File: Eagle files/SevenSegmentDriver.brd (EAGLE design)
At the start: 18.4 x 25.4 mm, 4 parts, among them IC1 74HC595D

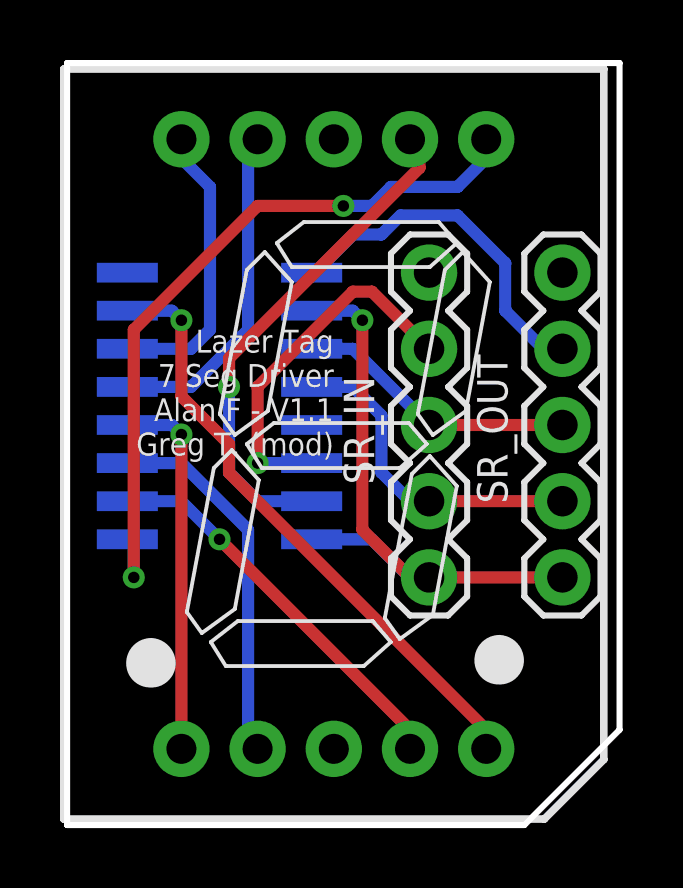
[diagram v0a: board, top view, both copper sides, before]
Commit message: Fixes
more fixes >:|
should e ready for fabbing
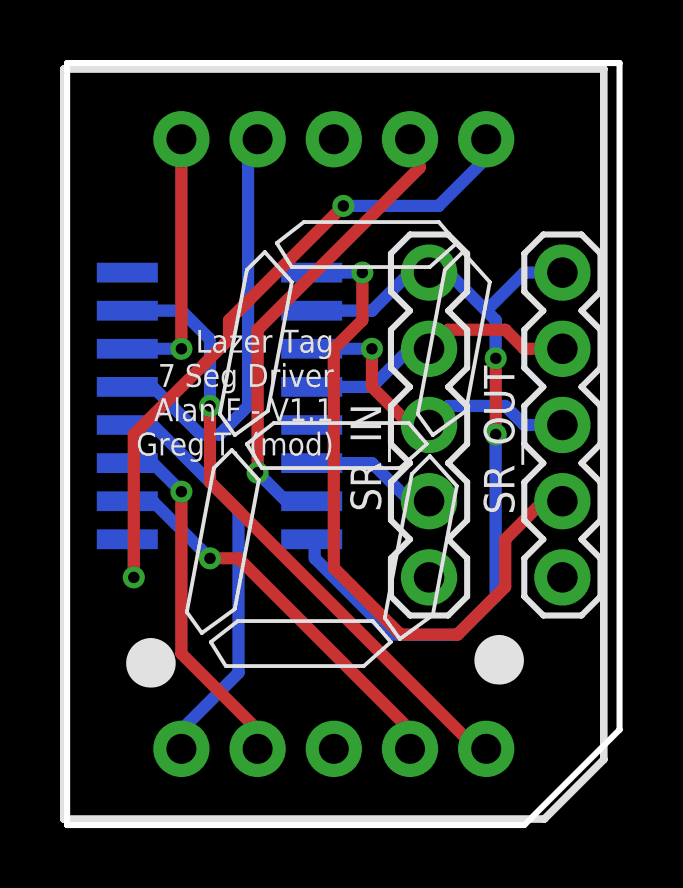
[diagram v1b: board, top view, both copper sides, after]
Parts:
- moved SR_IN 10.2 mm to (51.4, 37.5), turned to 270 degrees
- moved SR_OUT 10.2 mm to (55.9, 37.5), turned to 270 degrees
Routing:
- net SER_OUT: track 11.9 -> 23.2 mm, vias 0 -> 1
- net SER_IN: track 12.2 -> 4.44 mm, vias 1 -> 0
- net VCC: track 20.6 -> 27.9 mm, vias 1 -> 2
- net N$8: track 11.3 -> 14.1 mm
- net N$4: track 24.5 -> 22.8 mm
- net RCLK: track 11.1 -> 9.41 mm
- net N$3: track 17.0 -> 15.7 mm
- net SCLK: track 9.41 -> 10.7 mm, vias 0 -> 1
- net N$7: track 12.4 -> 13.6 mm, vias 1 -> 0
- net N$9: track 9.76 -> 8.79 mm, vias 0 -> 1
- net N$6: track 12.4 -> 11.8 mm, vias 0 -> 1
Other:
- board text removed: "RC"
- board text removed: "SI"
- board text removed: "SO"
- board text removed: "SR"
